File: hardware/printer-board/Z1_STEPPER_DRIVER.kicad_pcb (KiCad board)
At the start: 2 copper layers, 7 parts, among them J10 TO_MOTOR, J9 MS_SELECT, U6 A4988_MODULE

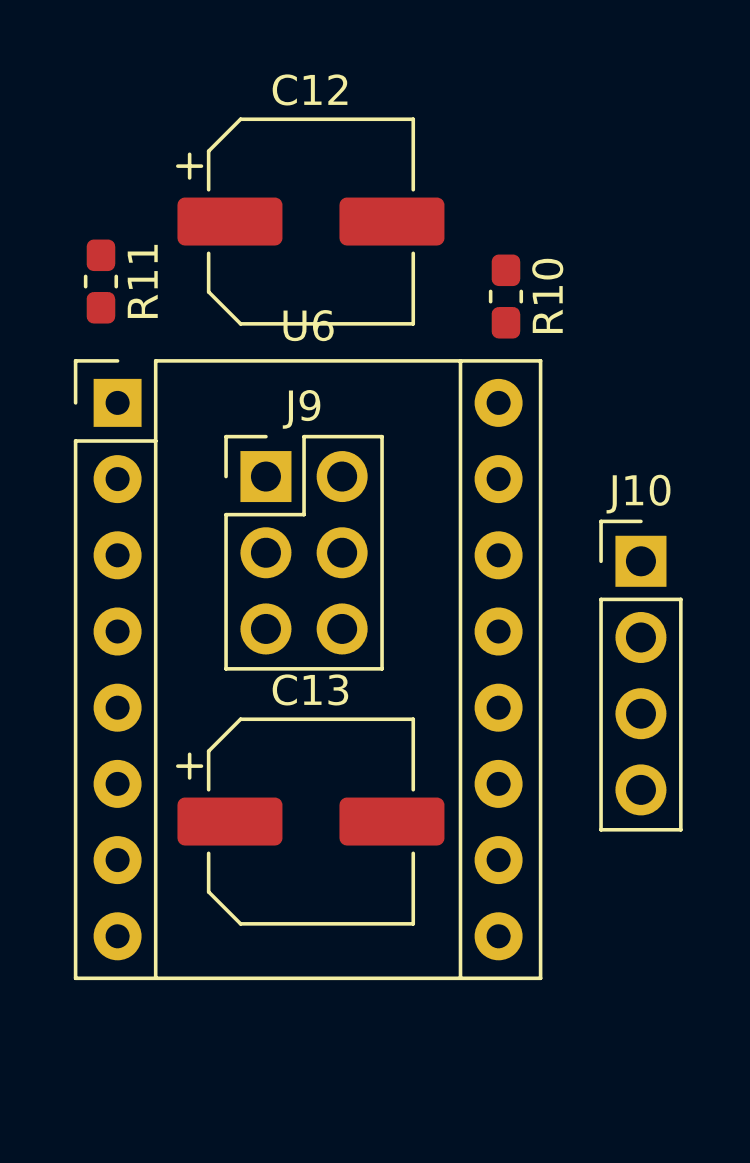
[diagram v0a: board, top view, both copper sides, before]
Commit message: update heater layouts,
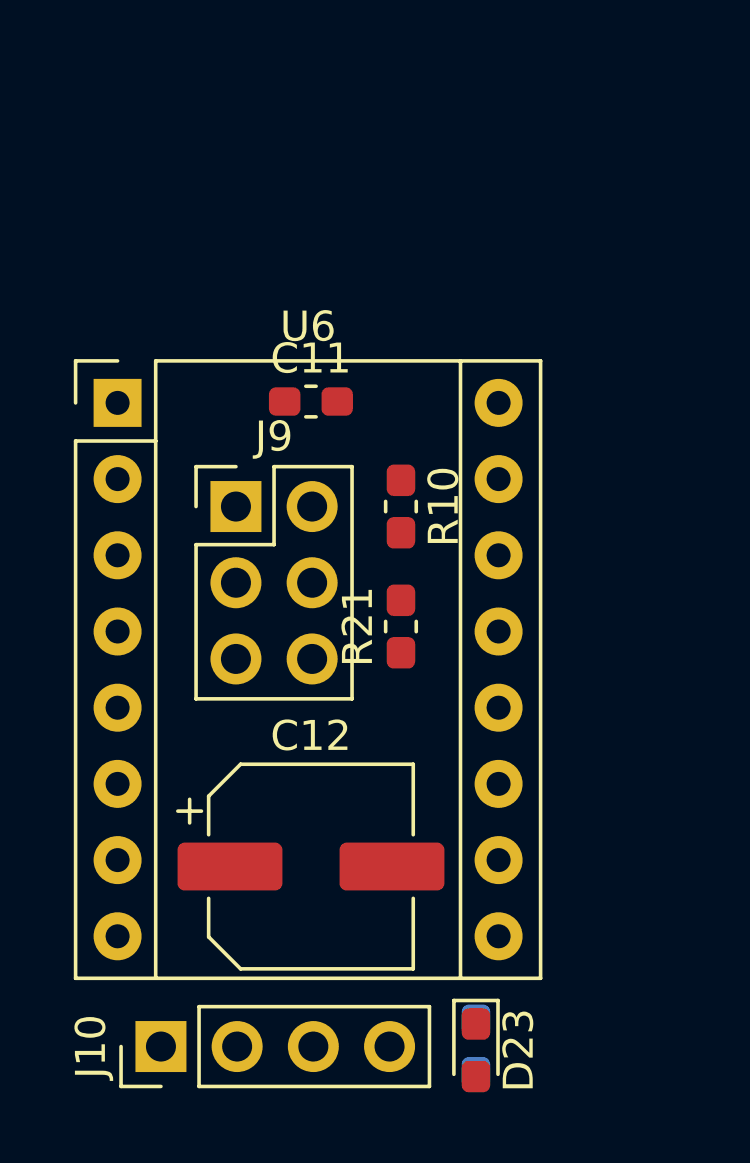
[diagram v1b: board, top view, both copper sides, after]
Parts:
- removed C13: CP100uf,25V, Capacitor_SMD:CP_Elec_6.3x7.7
- removed R11: R103,0603, Resistor_SMD:R_0603_1608Metric_Pad1.05x0.95mm_HandSolder
- added C11: C104,0603, Capacitor_SMD:C_0603_1608Metric_Pad1.05x0.95mm_HandSolder, F.Cu at (68.0, 36.5)
- added D23: LED_BLUE,0603, LED_SMD:LED_0603_1608Metric_Pad1.05x0.95mm_HandSolder, F.Cu at (73.5, 58.1)
- added R20: R102,0603, Resistor_SMD:R_0603_1608Metric_Pad1.05x0.95mm_HandSolder, B.Cu at (73.5, 58.0)
- added R21: R103,0603, Resistor_SMD:R_0603_1608Metric_Pad1.05x0.95mm_HandSolder, F.Cu at (71.0, 44.0)
- J10: value TO_MOTOR -> Z1
- moved J10 22.8 mm to (63.0, 58.0), turned to 90 degrees
- moved C12 21.5 mm to (68.0, 52.0)
- moved R10 7.83 mm to (71.0, 40.0)
- moved J9 1.41 mm to (65.5, 40.0)
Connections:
- net +5V renamed +3V3_STM32
- net /DIR renamed /Z1_DIR
- net /STEP renamed /Z1_STEP
- U6 pad 1: /~EN~ -> /~Z1_EN~
